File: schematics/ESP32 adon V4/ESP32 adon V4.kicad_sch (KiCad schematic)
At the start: 43 parts, among them J1 Conn_01x08_Pin, J10 Conn_01x01, J11 Conn_01x01, J12 Conn_01x01, J13 Conn_01x01, J14 Conn_01x01, J2 Conn_01x08_Pin, J3 Conn_01x02_Pin, J4 Conn_01x08_Pin, J5 Conn_01x08_Pin, J6 USB4215-03-A_REVA, J7 Conn_01x04_Pin, J9 Conn_01x04_Pin, Q1 MMBT7001K, Q2 MMBT7001K, Q3 MMBT7001K, SW2 SW_Push, U1 ESP32-C6-WROOM-1, U2 TCA9535DBR, U3 ADS1115IDGS, U4 TLV75733PDBV, U5 USBLC6-2SC6, U6 MLX90395KDC-BBA-101-RE

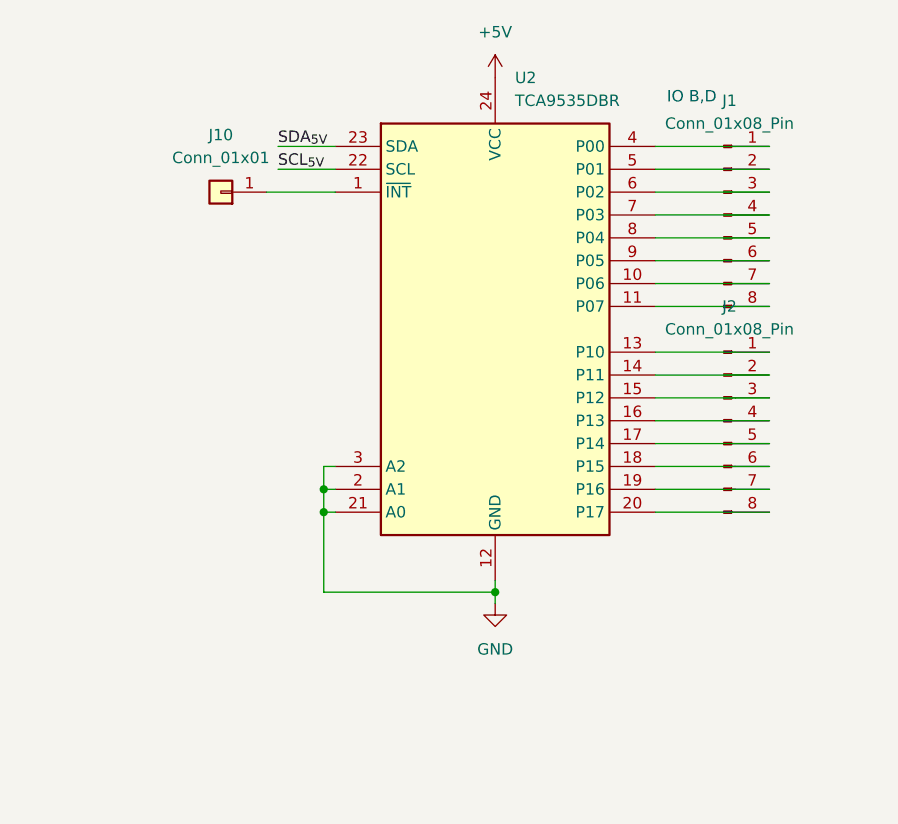
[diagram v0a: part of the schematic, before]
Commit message: update de ESP addon en de powerpoint
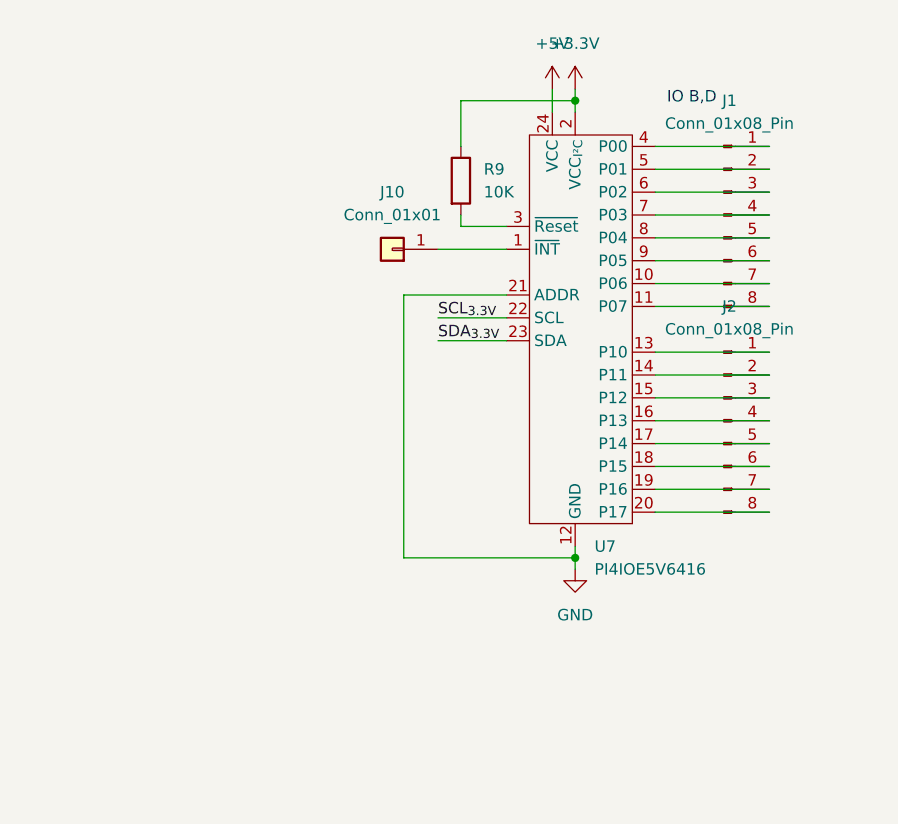
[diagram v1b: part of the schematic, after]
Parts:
- removed U2: TCA9535DBR, Package_SO:TSSOP-24_4.4x7.8mm_P0.65mm, symbol Interface_Expansion:TCA9535DBR
- added R9: 10K, Resistor_SMD:R_0603_1608Metric, symbol Device:R
- added U7: PI4IOE5V6416, Package_SO:TSSOP-24_4.4x7.8mm_P0.65mm, symbol robot:PI4IOE5V6416
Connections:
- net +3.3V: now also R9.1, U7.2 (VCC_{I²C})
- net +5V: now also U7.24 (VCC)
- net GND: now also U7.12 (GND), U7.21 (ADDR)
- net SCL_{3.3V}: now also U7.22 (SCL)
- net SDA_{3.3V}: now also U7.23 (SDA)
- net at J2.1 (Pin_1): now also U7.13 (P10)
- net at J2.2 (Pin_2): now also U7.14 (P11)
- net at J2.3 (Pin_3): now also U7.15 (P12)
- net at J2.4 (Pin_4): now also U7.16 (P13)
- net at J2.5 (Pin_5): now also U7.17 (P14)
- net at J2.6 (Pin_6): now also U7.18 (P15)
- net at J2.7 (Pin_7): now also U7.19 (P16)
- net at J2.8 (Pin_8): now also U7.20 (P17)
- net at J1.1 (Pin_1): now also U7.4 (P00)
- net at J1.2 (Pin_2): now also U7.5 (P01)
- net at J1.3 (Pin_3): now also U7.6 (P02)
- net at J1.4 (Pin_4): now also U7.7 (P03)
- net at J1.5 (Pin_5): now also U7.8 (P04)
- net at J1.6 (Pin_6): now also U7.9 (P05)
- net at J1.7 (Pin_7): now also U7.10 (P06)
- net at J1.8 (Pin_8): now also U7.11 (P07)
- net at J10.1 (Pin_1): now also U7.1 (~{INT})
- new net: R9.2, U7.3 (~{Reset})
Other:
- moved on the sheet: J10
